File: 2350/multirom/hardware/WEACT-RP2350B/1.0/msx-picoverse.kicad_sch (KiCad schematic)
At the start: 10 parts, among them J1 Micro_SD_Card, U1 WEACT-RP2350B

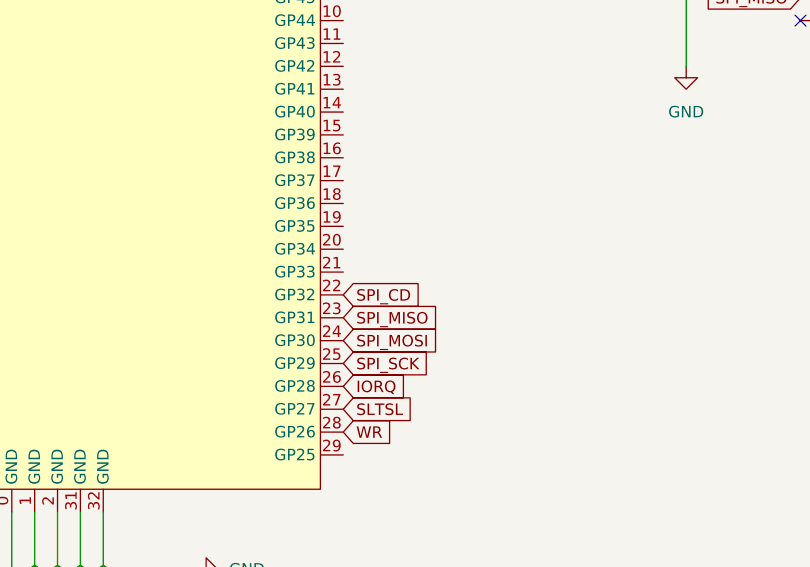
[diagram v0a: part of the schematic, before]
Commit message: playing with SPI libraries
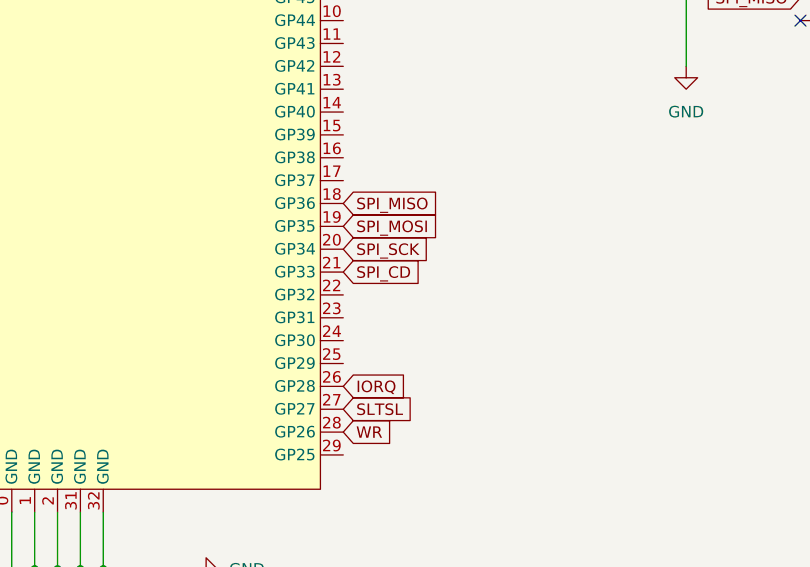
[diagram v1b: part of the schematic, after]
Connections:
- net SPI_CD: now also U1.21 (GP33); no longer U1.22 (GP32)
- net SPI_MISO: now also U1.18 (GP36); no longer U1.23 (GP31)
- net SPI_MOSI: now also U1.19 (GP35); no longer U1.24 (GP30)
- net SPI_SCK: now also U1.20 (GP34); no longer U1.25 (GP29)
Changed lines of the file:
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@@
 	(global_label "SPI_SCK"
 		(shape input)
-		(at 297.18 127 0)
-		(fields_autoplaced yes)
-		(effects
-			(font
-				(size 1.27 1.27)
-			)
-			(justify left)
-		)
-		(property "Intersheetrefs" "${INTERSHEET_REFS}"
-			(at 307.9666 127 0)
-			(effects
-				(font
-					(size 1.27 1.27)
-				)
-				(justify left)
-				(hide yes)
-			)
-		)
-	)
-	(global_label "SPI_SCK"
-		(shape input)
 		(at 347.98 81.28 180)
 		(fields_autoplaced yes)
@@
 		)
 	)
+	(global_label "A3"
+		(shape input)
+		(at 248.92 129.54 180)
+		(fields_autoplaced yes)
+		(effects
+			(font
+				(size 1.27 1.27)
+			)
+			(justify right)
+		)
+		(property "Intersheetrefs" "${INTERSHEET_REFS}"
+			(at 243.6367 129.54 0)
+			(effects
+				(font
+					(size 1.27 1.27)
+				)
+				(justify right)
+				(hide yes)
+			)
+		)
+	)
 	(global_label "SPI_CD"
 		(shape input)
-		(at 297.18 119.38 0)
-		(fields_autoplaced yes)
-		(effects
-			(font
-				(size 1.27 1.27)
-			)
-			(justify left)
-		)
-		(property "Intersheetrefs" "${INTERSHEET_REFS}"
-			(at 306.7571 119.38 0)
-			(effects
-				(font
-					(size 1.27 1.27)
-				)
-				(justify left)
-				(hide yes)
-			)
-		)
-	)
-	(global_label "A3"
-		(shape input)
-		(at 248.92 129.54 180)
-		(fields_autoplaced yes)
-		(effects
-			(font
-				(size 1.27 1.27)
-			)
-			(justify right)
-		)
-		(property "Intersheetrefs" "${INTERSHEET_REFS}"
-			(at 243.6367 129.54 0)
-			(effects
-				(font
-					(size 1.27 1.27)
-				)
-				(justify right)
+		(at 297.18 116.84 0)
+		(fields_autoplaced yes)
+		(effects
+			(font
+				(size 1.27 1.27)
+			)
+			(justify left)
+		)
+		(property "Intersheetrefs" "${INTERSHEET_REFS}"
+			(at 306.7571 116.84 0)
+			(effects
+				(font
+					(size 1.27 1.27)
+				)
+				(justify left)
 				(hide yes)
 			)
@@
 		)
 	)
+	(global_label "SPI_MISO"
+		(shape input)
+		(at 297.18 109.22 0)
+		(fields_autoplaced yes)
+		(effects
+			(font
+				(size 1.27 1.27)
+			)
+			(justify left)
+		)
+		(property "Intersheetrefs" "${INTERSHEET_REFS}"
+			(at 308.8133 109.22 0)
+			(effects
+				(font
+					(size 1.27 1.27)
+				)
+				(justify left)
+				(hide yes)
+			)
+		)
+	)
 	(global_label "RD"
 		(shape input)
@@
 		)
 	)
+	(global_label "SPI_SCK"
+		(shape input)
+		(at 297.18 114.3 0)
+		(fields_autoplaced yes)
+		(effects
+			(font
+				(size 1.27 1.27)
+			)
+			(justify left)
+		)
+		(property "Intersheetrefs" "${INTERSHEET_REFS}"
+			(at 307.9666 114.3 0)
+			(effects
+				(font
+					(size 1.27 1.27)
+				)
+				(justify left)
+				(hide yes)
+			)
+		)
+	)
 	(global_label "A10"
 		(shape input)
@@
 				)
 				(justify right)
+				(hide yes)
+			)
+		)
+	)
+	(global_label "SPI_MOSI"
+		(shape input)
+		(at 297.18 111.76 0)
+		(fields_autoplaced yes)
+		(effects
+			(font
+				(size 1.27 1.27)
+			)
+			(justify left)
+		)
+		(property "Intersheetrefs" "${INTERSHEET_REFS}"
+			(at 308.8133 111.76 0)
+			(effects
+				(font
+					(size 1.27 1.27)
+				)
+				(justify left)
 				(hide yes)
 			)
@@
 		)
 	)
-	(global_label "SPI_MOSI"
-		(shape input)
-		(at 297.18 124.46 0)
-		(fields_autoplaced yes)
-		(effects
-			(font
-				(size 1.27 1.27)
-			)
-			(justify left)
-		)
-		(property "Intersheetrefs" "${INTERSHEET_REFS}"
-			(at 308.8133 124.46 0)
-			(effects
-				(font
-					(size 1.27 1.27)
-				)
-				(justify left)
-				(hide yes)
-			)
-		)
-	)
 	(global_label "WR"
 		(shape input)
@@
 			(effects
 				(font
-					(size 1.27 1.27)
-				)
-				(justify left)
-				(hide yes)
-			)
-		)
-	)
-	(global_label "SPI_MISO"
-		(shape input)
-		(at 297.18 121.92 0)
-		(fields_autoplaced yes)
-		(effects
-			(font
-				(size 1.27 1.27)
-			)
-			(justify left)
-		)
-		(property "Intersheetrefs" "${INTERSHEET_REFS}"
-			(at 308.8133 121.92 0)
-			(effects
-				(font
